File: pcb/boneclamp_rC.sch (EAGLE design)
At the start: 163 parts, among them IC1 24C, IC2 LM741D, IC3 LM741D, U1 AD8032ARZ-REEL7, U10 ADA4841-2YRZ, U11 ADA4841-2YRZ, U12 ADS8331IBPW, U13 OPA365AIDBVR, U14 REF5040MDREP, U15 OPA365AIDBVR, U16 OPA365AIDBVR, U2 LT1964ES5-5TRMPBF, U3 OPA365AIDBVR, U4 TLV70245DBVT, U5 ADA4841-2YRZ, U6 AD713JRZ-16, U8 TPS63700DRCT, U9 ADA4841-2YRZ

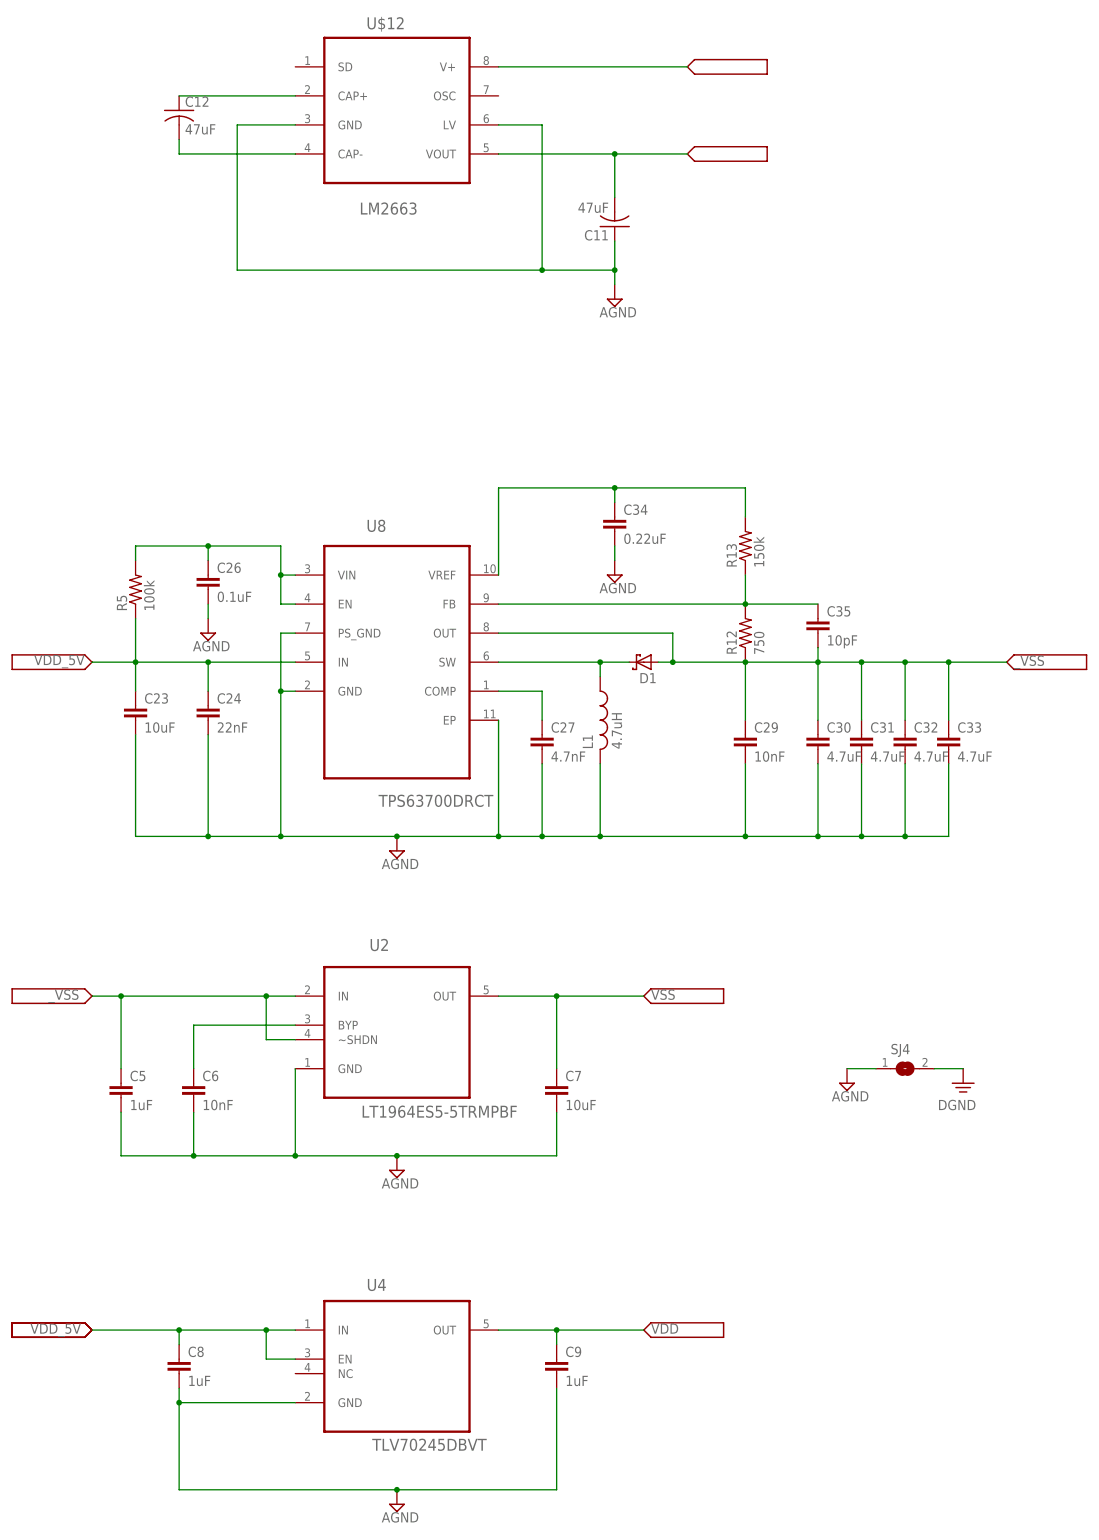
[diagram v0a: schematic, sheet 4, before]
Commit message: Minor changes.
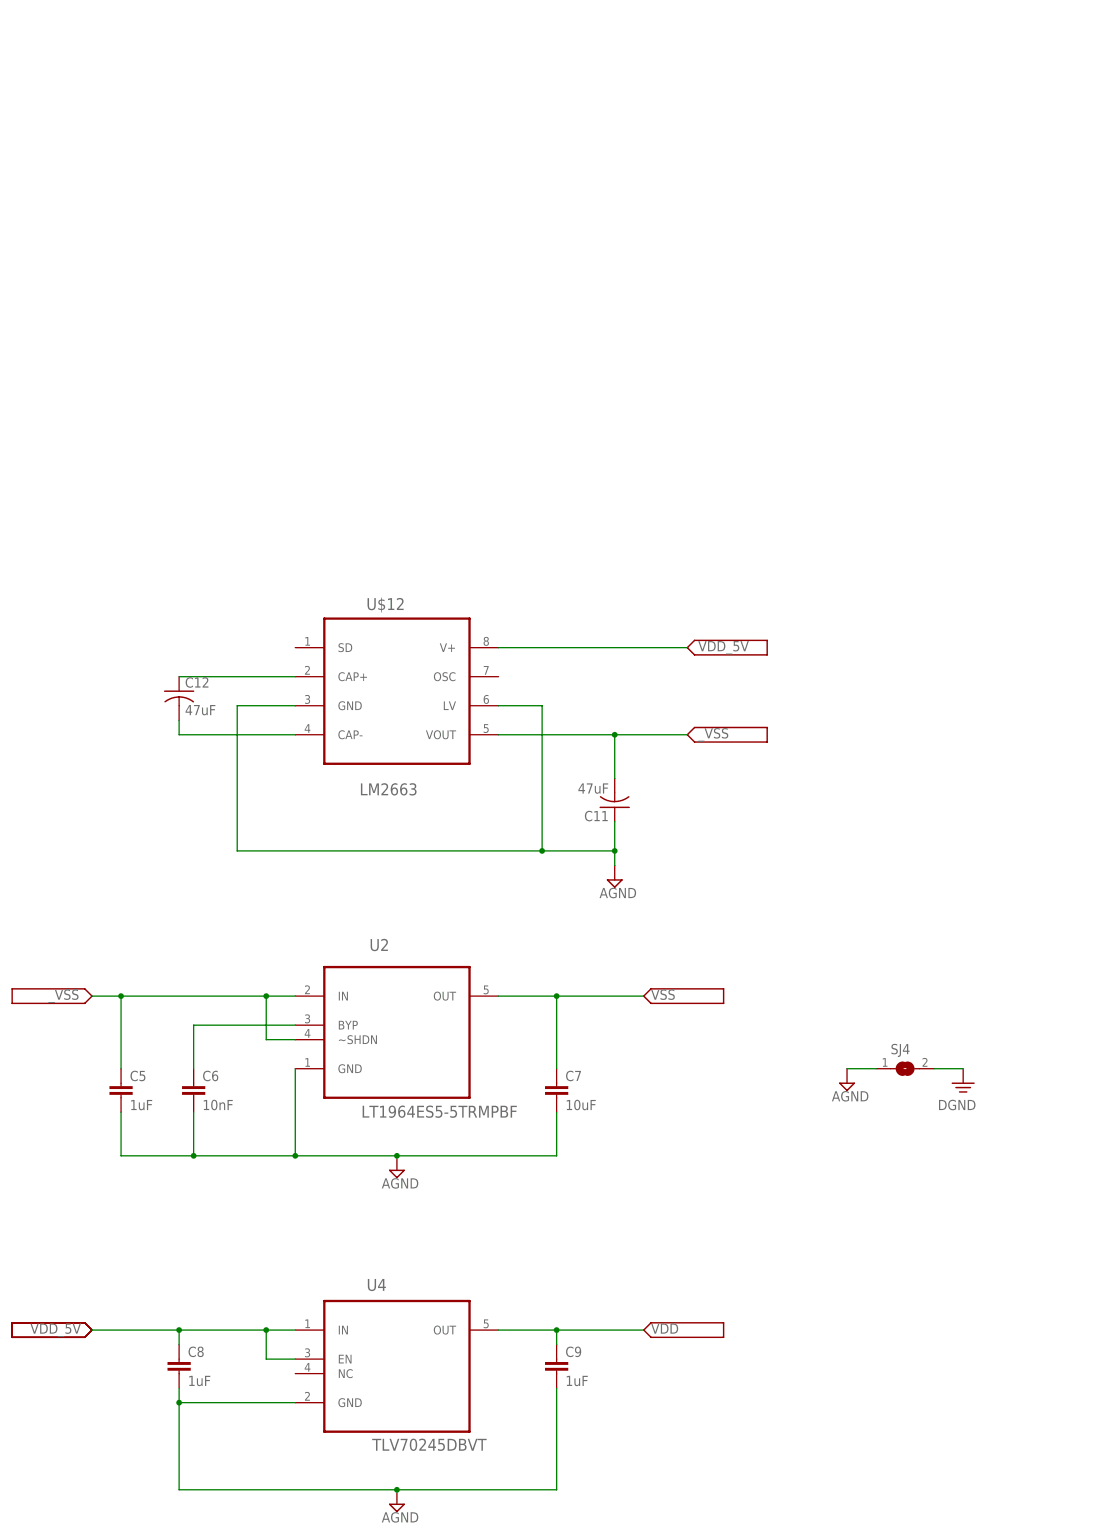
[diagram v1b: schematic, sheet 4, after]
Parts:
- removed C23: 10uF, rcl:C-EUC0603
- removed C24: 22nF, rcl:C-EUC0603
- removed C26: 0.1uF, rcl:C-EUC0603
- removed C27: 4.7nF, rcl:C-EUC0603
- removed C29: 10nF, rcl:C-EUC0603
- removed C30, C31, C32, C33: 4.7uF, rcl:C-EUC0603
- removed C34: 0.22uF, rcl:C-EUC0603
- removed C35: 10pF, rcl:C-EUC0603
- removed D1: SCHOTTKY-DIODE-2, boneclamp:SCHOTTKY-DIODE-2
- removed L1: 4.7uH, boneclamp:L-US
- removed R12: 750, rcl:R-US_R0603
- removed R13: 150k, rcl:R-US_R0603
- removed R5: 100k, rcl:R-US_R0603
- removed U8: TPS63700DRCT, ti-extended:TPS63700DRCT
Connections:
- removed net N$23: C26.1, R5.2, U8.EN, U8.VIN
- removed net N$25: C27.1, U8.COMP
- removed net N$27: D1.A, L1.1, U8.SW
- removed net N$30: C35.1, R12.2, R13.1, U8.FB
- removed net N$31: C34.1, R13.2, U8.VREF
- net AGND: no longer C23.2, C24.2, C26.2, C27.2, C29.2, C30.2, C31.2, C32.2, C33.2, C34.2, L1.2, U8.EP, U8.GND, U8.PS_GND
- net VDD_5V: no longer C23.1, C24.1, R5.1, U8.IN
- net _VSS: no longer C29.1, C30.1, C31.1, C32.1, C33.1, C35.2, D1.C, R12.1, U8.OUT
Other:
- moved on the sheet: C11, C12, U$12
